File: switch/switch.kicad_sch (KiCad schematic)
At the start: 26 parts, among them J1 1935174, J2 1935174, K1 ASO242, Q1 SFH309, Q2 BC847

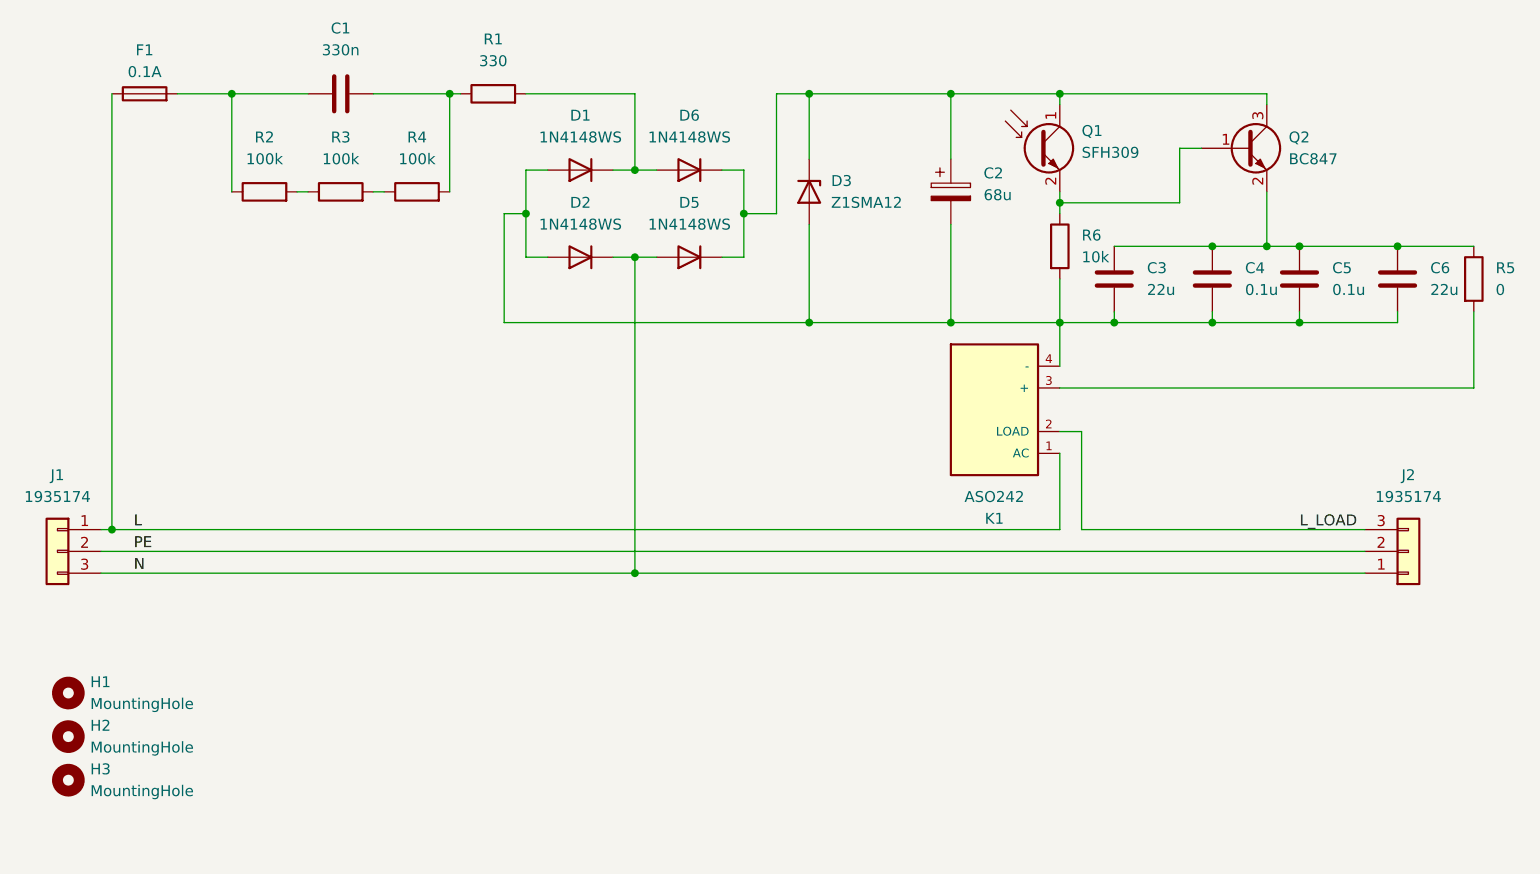
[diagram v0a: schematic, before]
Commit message: Updated rev
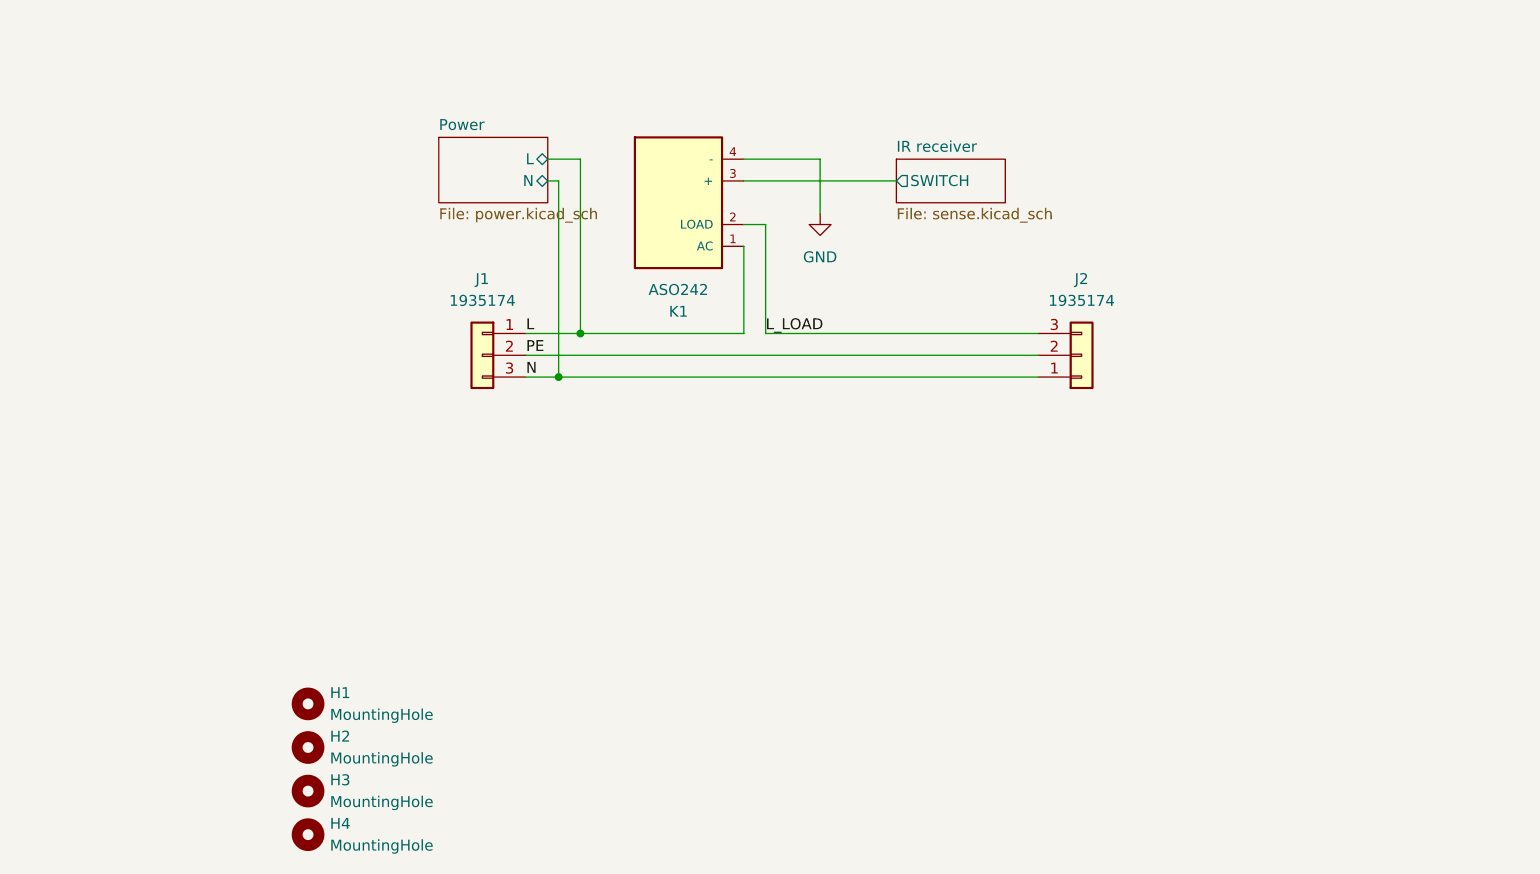
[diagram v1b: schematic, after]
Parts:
- removed C1: 330n, Capacitor_THT:C_Rect_L24.0mm_W7.0mm_P22.50mm_MKT, symbol Device:C
- removed C2: 68u, Capacitor_SMD:CP_Elec_10x12.5, symbol Device:C_Polarized
- removed C3, C6: 22u, Capacitor_SMD:C_1210_3225Metric, symbol Device:C
- removed C4, C5: 0.1u, Capacitor_SMD:C_0603_1608Metric, symbol Device:C
- removed D1, D2, D5, D6: 1N4148WS, Diode_SMD:D_SOD-323_HandSoldering, symbol Diode:1N4148WS
- removed D3: Z1SMA12, Diode_SMD:D_SMA, symbol Diode:Z1SMAxxx
- removed F1: 0.1A, Capacitor_THT:C_Disc_D8.0mm_W5.0mm_P5.00mm, symbol Device:Fuse
- removed Q1: SFH309, LED_THT:LED_D3.0mm_Clear, symbol Sensor_Optical:SFH309
- removed Q2: BC847, Package_TO_SOT_SMD:SOT-23, symbol Transistor_BJT:BC847
- removed R1: 330, Resistor_THT:R_Axial_DIN0516_L15.5mm_D5.0mm_P7.62mm_Vertical, symbol Device:R
- removed R2, R3, R4: 100k, Resistor_SMD:R_0805_2012Metric, symbol Device:R
- removed R5: 0, Resistor_SMD:R_0603_1608Metric, symbol Device:R
- removed R6: 10k, Resistor_SMD:R_0805_2012Metric, symbol Device:R
- added H4: MountingHole, MountingHole:MountingHole_2.2mm_M2_DIN965, symbol Mechanical:MountingHole
- K1: MPN1 (none) -> Sensata:ASO242; SKU1 (none) -> Conrad:188012
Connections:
- net GND: now reaches K1.4 (-)
- net IR receiver/SWITCH: now reaches K1.3 (+)
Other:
- added sheet IR receiver (sense.kicad_sch)
- added sheet Power (power.kicad_sch)
- moved on the sheet: H1, H2, H3, J1, J2, K1
